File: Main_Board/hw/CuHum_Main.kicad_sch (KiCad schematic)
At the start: 50 parts, among them J1 Barrel_Jack_Switch_Pin3Ring, J101 Conn_01x07, J102 Conn_01x07, J103 Conn_01x07, J104 Conn_01x07, J105 Conn_01x07, J106 Conn_01x07, J107 Conn_01x07, J108 Conn_01x07, J109 Conn_01x07, J110 Conn_01x07, J111 Conn_01x07, J112 Conn_01x07, J113 Conn_01x07, J114 Conn_01x07, J115 Conn_01x07, J2 Conn_01x04, U1 MT2492, U2 STM32G030K6Tx, U3 MAX98357AETE+, U4 W25Q16JVSS, U5 MPR121QR2, U6 MPR121QR2, X1 12.288MHz

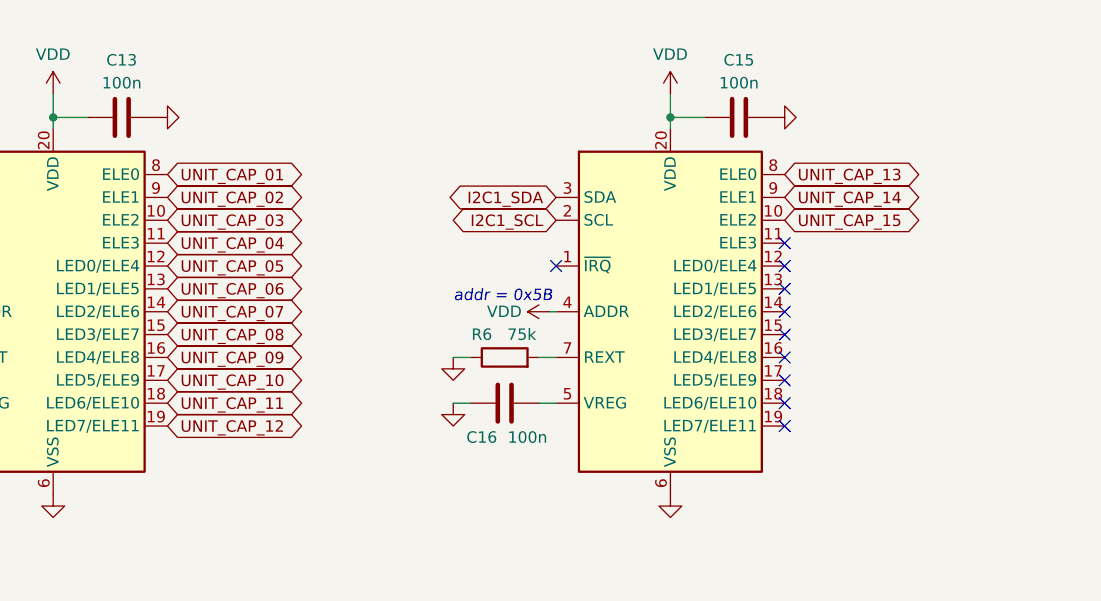
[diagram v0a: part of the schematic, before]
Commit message: (WIP) Main board layout & routing
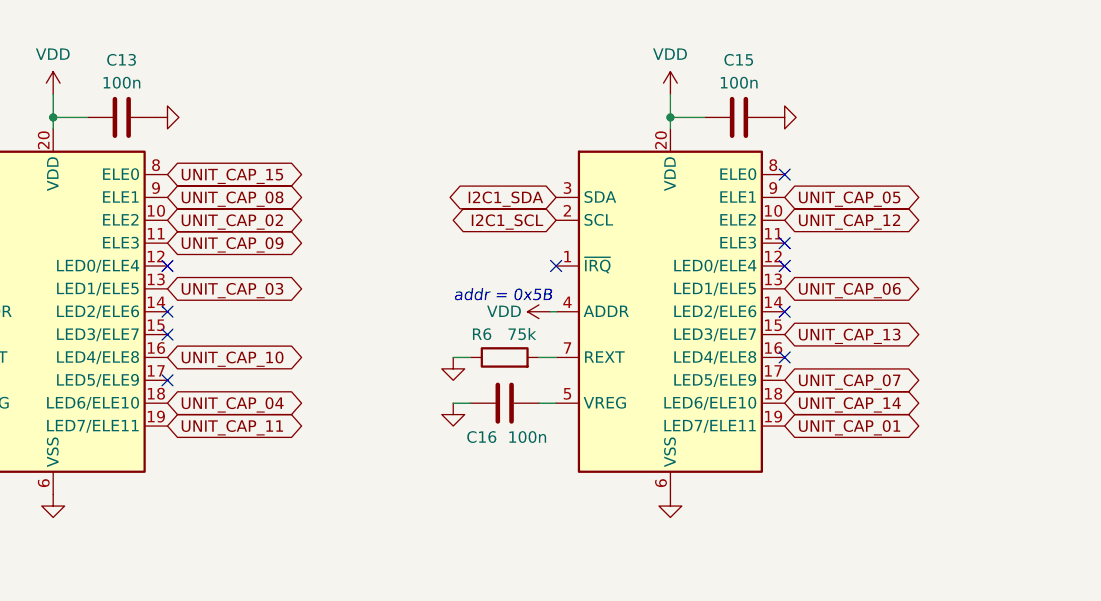
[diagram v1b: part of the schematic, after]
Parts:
- J101, J102, J103, J104, J105, J106, J107, J108, J109, J110, J111, J112, J113, J114, J115: footprint Connector_PinHeader_2.54mm:PinHeader_1x07_P2.54mm_Vertical -> CuHum_Main_footprints:Unit_1x07_P2.54
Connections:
- net UNIT_CAP_01: now also U6.19 (LED7/ELE11); no longer U5.8 (ELE0)
- net UNIT_CAP_02: now also U5.10 (ELE2); no longer U5.9 (ELE1)
- net UNIT_CAP_03: now also U5.13 (LED1/ELE5); no longer U5.10 (ELE2)
- net UNIT_CAP_04: now also U5.18 (LED6/ELE10); no longer U5.11 (ELE3)
- net UNIT_CAP_05: now also U6.9 (ELE1); no longer U5.12 (LED0/ELE4)
- net UNIT_CAP_06: now also U6.13 (LED1/ELE5); no longer U5.13 (LED1/ELE5)
- net UNIT_CAP_07: now also U6.17 (LED5/ELE9); no longer U5.14 (LED2/ELE6)
- net UNIT_CAP_08: now also U5.9 (ELE1); no longer U5.15 (LED3/ELE7)
- net UNIT_CAP_09: now also U5.11 (ELE3); no longer U5.16 (LED4/ELE8)
- net UNIT_CAP_10: now also U5.16 (LED4/ELE8); no longer U5.17 (LED5/ELE9)
- net UNIT_CAP_11: now also U5.19 (LED7/ELE11); no longer U5.18 (LED6/ELE10)
- net UNIT_CAP_12: now also U6.10 (ELE2); no longer U5.19 (LED7/ELE11)
- net UNIT_CAP_13: now also U6.15 (LED3/ELE7); no longer U6.8 (ELE0)
- net UNIT_CAP_14: now also U6.18 (LED6/ELE10); no longer U6.9 (ELE1)
- net UNIT_CAP_15: now also U5.8 (ELE0); no longer U6.10 (ELE2)
